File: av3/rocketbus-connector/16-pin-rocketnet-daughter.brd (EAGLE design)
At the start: 20.2 x 8 mm, 1 part

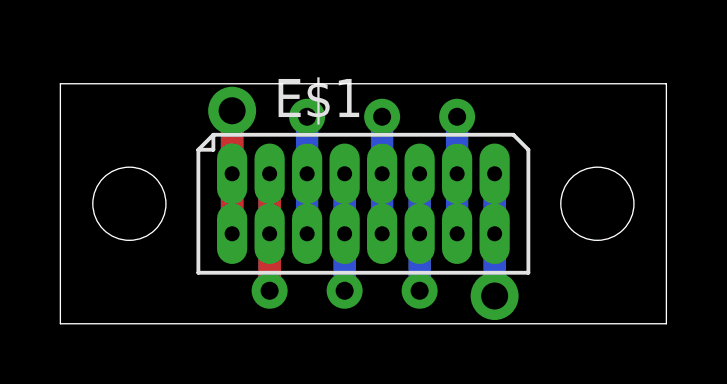
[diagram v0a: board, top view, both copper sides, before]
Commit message: Doh! Forgot to put wires on both sides of the board.
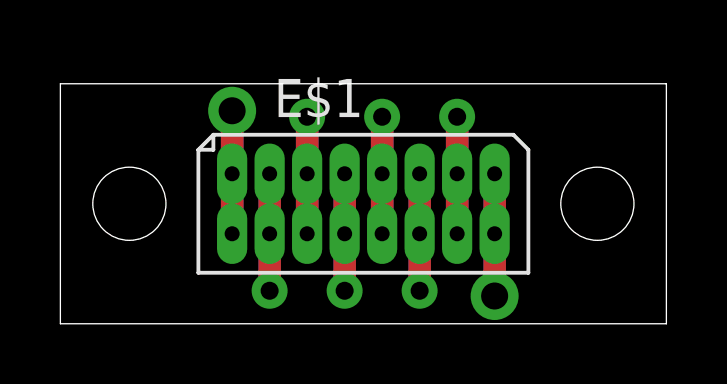
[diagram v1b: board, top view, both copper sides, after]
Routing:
- net B-: track 4.05 -> 8.15 mm, vias 0 -> 1
- net TX-: track 3.90 -> 7.83 mm
- net RX-: track 3.90 -> 7.80 mm, vias 0 -> 1
- net AUX2: track 3.90 -> 7.80 mm, vias 0 -> 1
- net RX+: track 3.90 -> 7.80 mm, vias 0 -> 1
- net AUX1: track 3.90 -> 7.80 mm, vias 0 -> 1
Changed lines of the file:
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@@
 <contactref element="E$1" pad="AUX2@14"/>
 <wire x1="13.225" y1="3" x2="13.225" y2="6.9" width="0.75" layer="16"/>
+<via x="13.225" y="6.9" extent="1-16" drill="0.6" diameter="1.2"/>
+<wire x1="13.225" y1="3" x2="13.225" y2="6.9" width="0.75" layer="1"/>
 </signal>
 <signal name="AUX1">
 <contactref element="E$1" pad="AUX1@11"/>
 <wire x1="11.975" y1="5" x2="11.975" y2="1.1" width="0.75" layer="16"/>
+<via x="11.975" y="1.1" extent="1-16" drill="0.6" diameter="1.2"/>
+<wire x1="11.975" y1="5" x2="11.975" y2="1.1" width="0.75" layer="1"/>
 </signal>
 <signal name="USB1_L">
@@
 <via x="8.225" y="6.9" extent="1-16" drill="0.6" diameter="1.2"/>
 </signal>
-<signal name="S$4">
-<via x="9.475" y="1.1" extent="1-16" drill="0.6" diameter="1.2"/>
-</signal>
-<signal name="S$5">
-<via x="10.725" y="6.9" extent="1-16" drill="0.6" diameter="1.2"/>
-</signal>
-<signal name="S$6">
-<via x="11.975" y="1.1" extent="1-16" drill="0.6" diameter="1.2"/>
-</signal>
-<signal name="S$7">
-<via x="13.225" y="6.9" extent="1-16" drill="0.6" diameter="1.2"/>
-</signal>
-<signal name="S$8">
-<via x="14.475" y="0.925" extent="1-16" drill="0.9" diameter="1.6"/>
-</signal>
 <signal name="TX+">
 <contactref element="E$1" pad="TX+@3"/>
@@
 <contactref element="E$1" pad="TX-@6"/>
 <wire x1="8.225" y1="3" x2="8.225" y2="6.9" width="0.75" layer="16"/>
+<wire x1="8.225" y1="3" x2="8.225" y2="6.925" width="0.75" layer="1"/>
 </signal>
 <signal name="RX+">
 <contactref element="E$1" pad="RX+@7"/>
 <wire x1="9.475" y1="5" x2="9.475" y2="1.1" width="0.75" layer="16"/>
+<via x="9.475" y="1.1" extent="1-16" drill="0.6" diameter="1.2"/>
+<wire x1="9.475" y1="5" x2="9.475" y2="1.1" width="0.75" layer="1"/>
 </signal>
 <signal name="RX-">
 <contactref element="E$1" pad="RX-@10"/>
 <wire x1="10.725" y1="3" x2="10.725" y2="6.9" width="0.75" layer="16"/>
+<via x="10.725" y="6.9" extent="1-16" drill="0.6" diameter="1.2"/>
+<wire x1="10.725" y1="3" x2="10.725" y2="6.9" width="0.75" layer="1"/>
 </signal>
 <signal name="B-">
 <contactref element="E$1" pad="B-@15"/>
-<wire x1="14.475" y1="5" x2="14.475" y2="0.95" width="0.75" layer="16"/>
+<via x="14.475" y="0.925" extent="1-16" drill="0.9" diameter="1.6"/>
+<wire x1="14.475" y1="5" x2="14.475" y2="0.925" width="0.75" layer="1"/>
+<wire x1="14.475" y1="5" x2="14.475" y2="0.925" width="0.75" layer="16"/>
 </signal>
 </signals>
